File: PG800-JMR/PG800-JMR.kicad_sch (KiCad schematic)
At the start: 49 parts, among them J1 DIN-6, J10 POT_POWER_2, J11 POT_POWER_3, J12 POT_POWER_4, J13 POT_CENTERS_4, J14 3.3V_BUS, J15 5V, J16 3.3V_ONBOARD_JUMPER, J2 POT_CENTERS_1, J3 POT_CENTERS_2, J4 POT_CENTERS_3, J5 TEENSY_PIN_BLK2, J6 TEENSY_PIN_BLK1, J7 TEENSY_PIN_BLK3, J8 GROUNDS, J9 POT_POWER_1, Q1 BSS138, Q2 BSS138, Q3 BSS138, U1 LM2575-5BT, U2 CD74HC4067M, U3 CD74HC4067M, U4 CD74HC4067M, U5 3.3V_REGULATOR_EXTERNAL, U6 CD74HC4067M

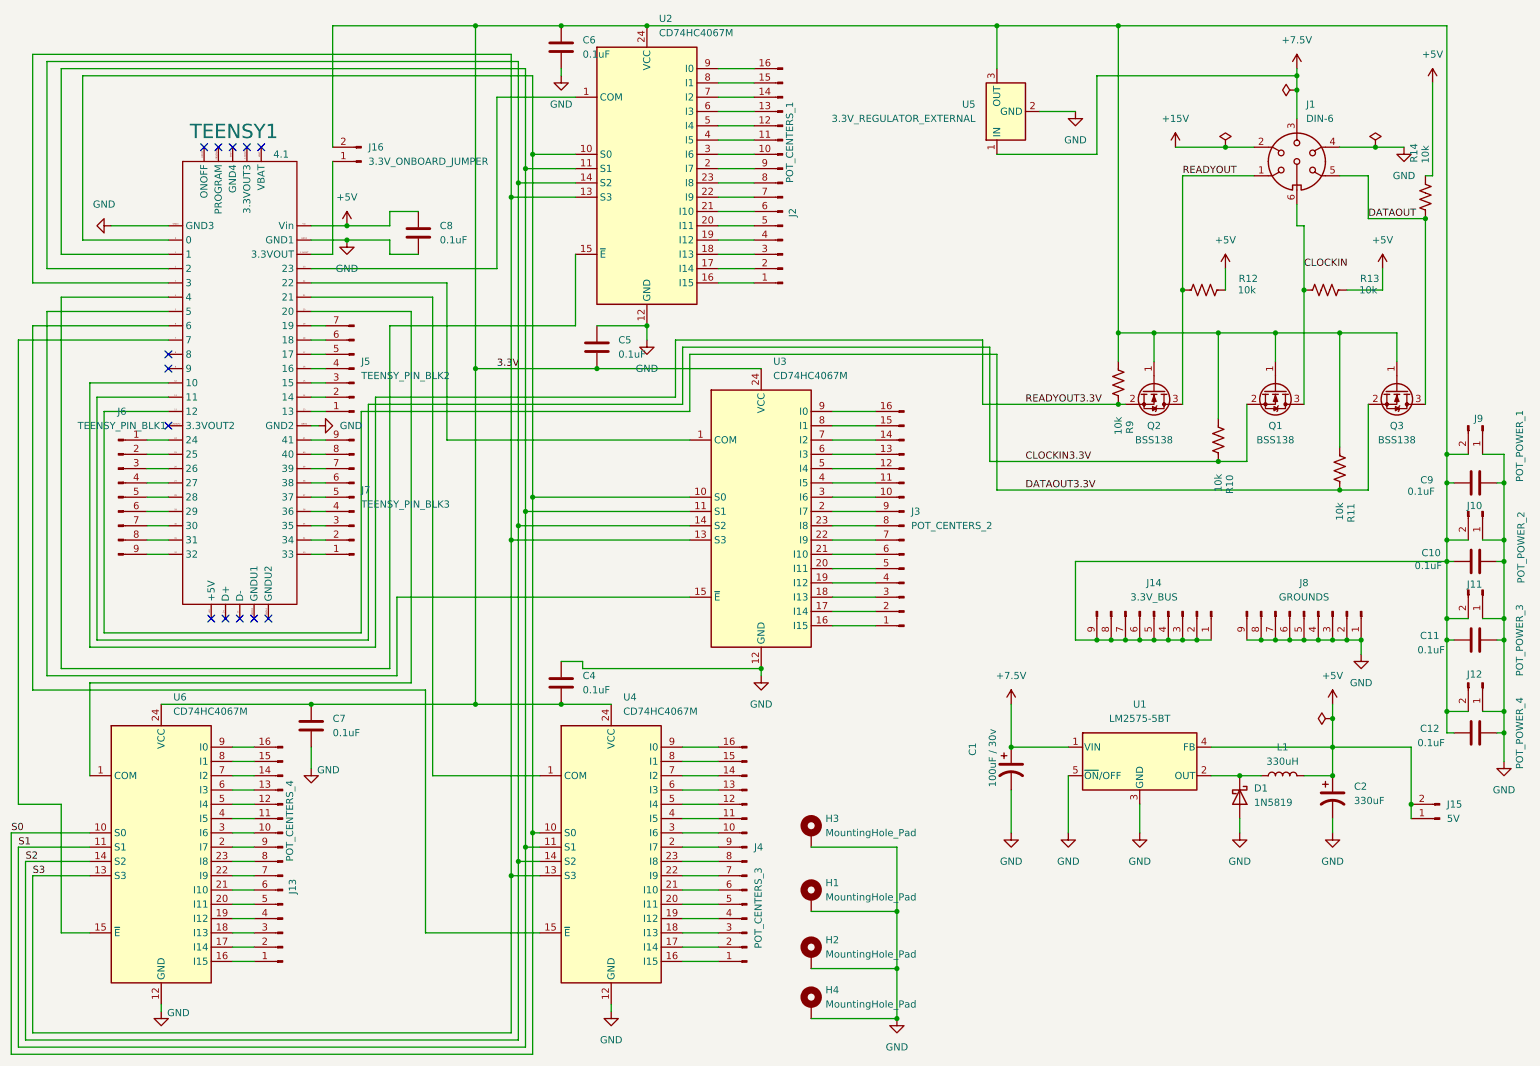
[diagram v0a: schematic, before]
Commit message: updated 3d image
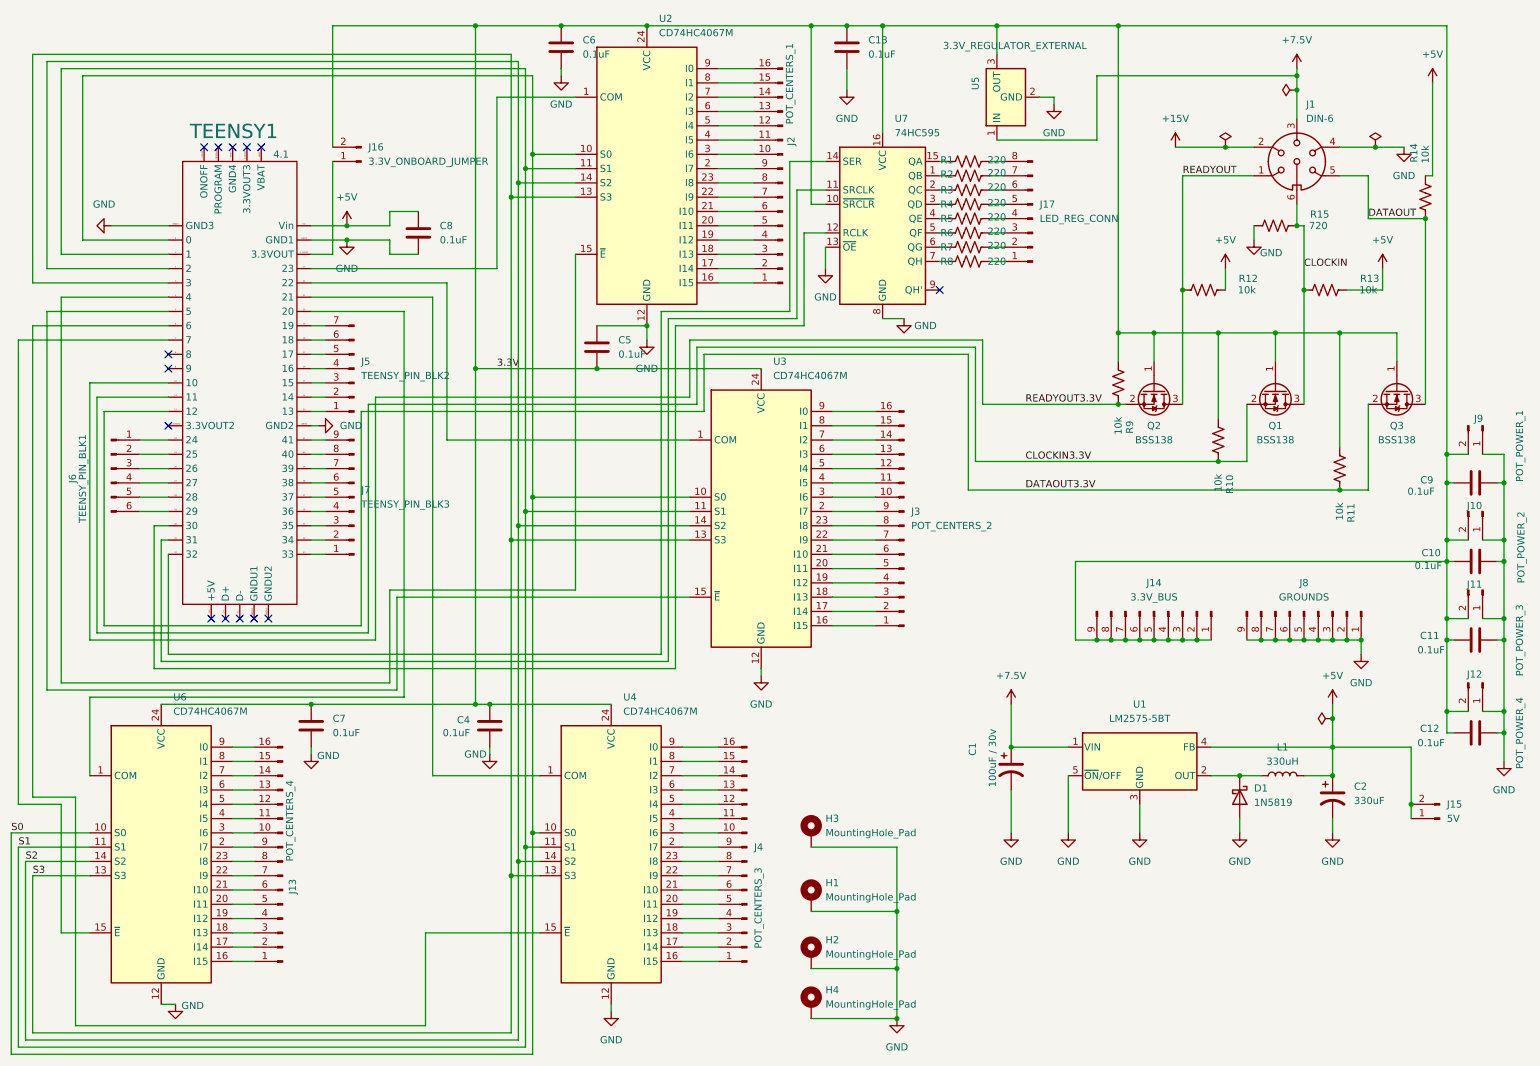
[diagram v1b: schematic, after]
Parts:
- removed J6: TEENSY_PIN_BLK1, Connector_PinHeader_2.54mm:PinHeader_1x09_P2.54mm_Vertical, symbol Connector:Conn_01x09_Pin
- added C13: 0.1uF, Capacitor_THT:C_Disc_D5.0mm_W2.5mm_P2.50mm, symbol Device:C
- added J17: LED_REG_CONN, Connector_PinHeader_2.54mm:PinHeader_1x08_P2.54mm_Vertical, symbol Connector:Conn_01x08_Pin
- added J6: TEENSY_PIN_BLK1, Connector_PinHeader_2.54mm:PinHeader_1x06_P2.54mm_Vertical, symbol Connector:Conn_01x06_Pin
- added R1, R2, R3, R4, R5, R6, R7, R8: 220, Resistor_THT:R_Axial_DIN0204_L3.6mm_D1.6mm_P2.54mm_Vertical, symbol Device:R_US
- added R15: 720, Resistor_THT:R_Axial_DIN0204_L3.6mm_D1.6mm_P2.54mm_Vertical, symbol Device:R_US
- added U7: 74HC595, Package_DIP:DIP-16_W7.62mm, symbol 74xx:74HC595
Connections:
- net 3.3V: now also C4.1, C13.1, U7.10 (~{SRCLR}), U7.16 (VCC); no longer C4.2
- net CLOCKIN: now also R15.1
- net GND: now also C4.2, C13.2, R15.2, U7.13 (~{OE}), U7.8 (GND); no longer C4.1
- net at TEENSY1.24: now also J6.1 (Pin_1)
- net at TEENSY1.25: now also J6.2 (Pin_2)
- net at TEENSY1.26: now also J6.3 (Pin_3)
- net at TEENSY1.27: now also J6.4 (Pin_4)
- net at TEENSY1.28: now also J6.5 (Pin_5)
- net at TEENSY1.29: now also J6.6 (Pin_6)
- net at TEENSY1.30: now also U7.12 (RCLK)
- net at TEENSY1.31: now also U7.11 (SRCLK)
- net at TEENSY1.32: now also U7.14 (SER)
- new net: R5.1, U7.4 (QE)
- new net: J17.4 (Pin_4), R5.2
- new net: R1.1, U7.15 (QA)
- new net: J17.8 (Pin_8), R1.2
- new net: R2.1, U7.1 (QB)
- new net: J17.7 (Pin_7), R2.2
- new net: R6.1, U7.5 (QF)
- new net: J17.3 (Pin_3), R6.2
- new net: R7.1, U7.6 (QG)
- new net: J17.2 (Pin_2), R7.2
- new net: R3.1, U7.2 (QC)
- new net: J17.6 (Pin_6), R3.2
- new net: R4.1, U7.3 (QD)
- new net: R8.1, U7.7 (QH)
- new net: J17.1 (Pin_1), R8.2
- new net: J17.5 (Pin_5), R4.2
- no-connect marks 13 -> 14
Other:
- moved on the sheet: C4, U5
